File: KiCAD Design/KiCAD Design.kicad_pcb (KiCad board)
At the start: 2 copper layers, 51 x 60.5 mm, 60 parts, among them J1 USB_B_Micro, J2 Conn_01x04_Pin, J5 Micro_SD_Card, SW1 SW_SPDT, U1 STM32F103C8Tx, U2 AMS1117-3.3, U3 BNO055, U4 L80-R, U5 nRF24L01P, Y1 16MHz, Y2 16MHz

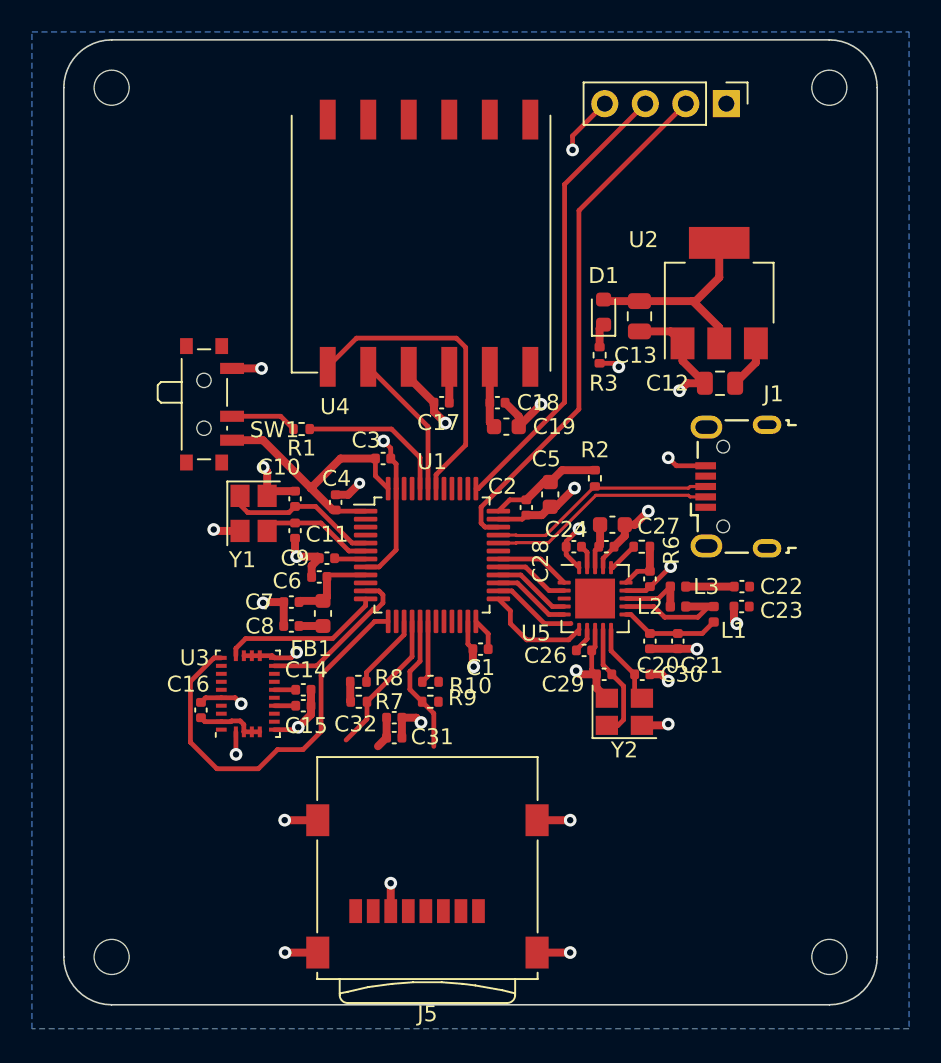
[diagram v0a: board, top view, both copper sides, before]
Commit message: All layout finished, ready to prep for order
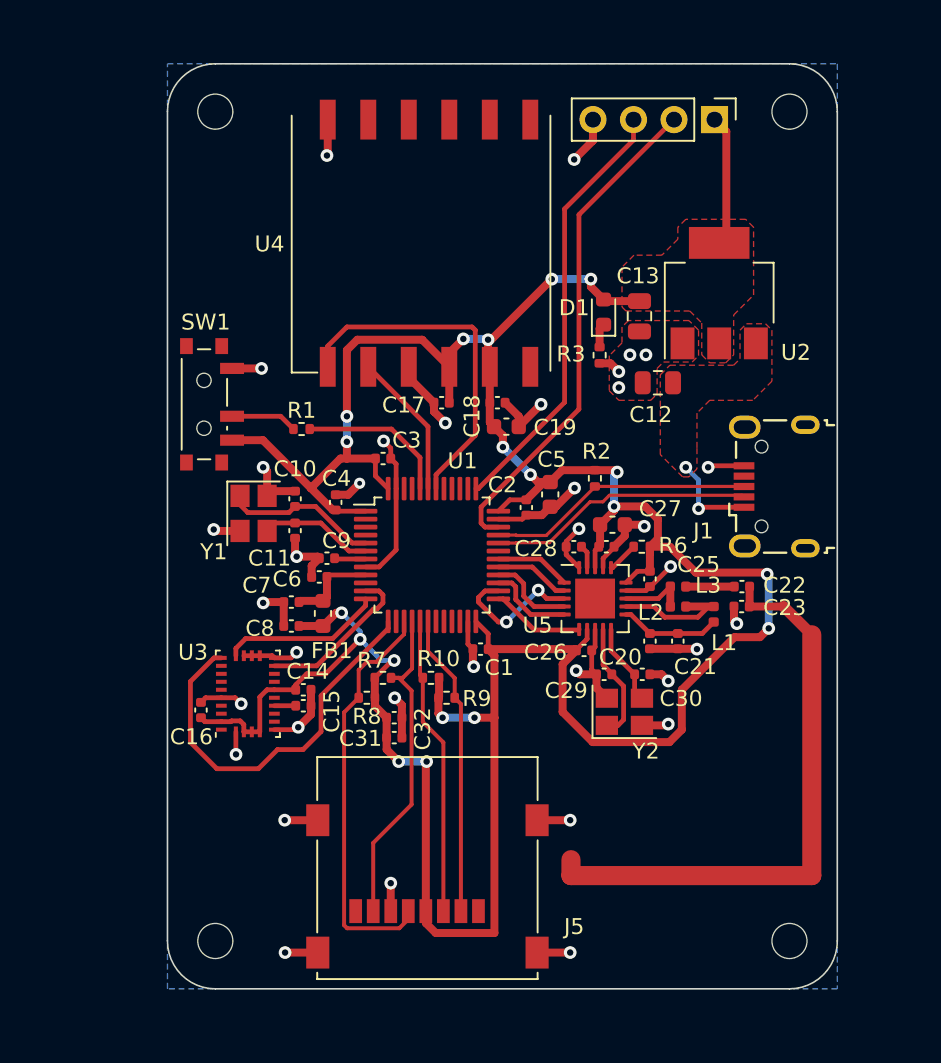
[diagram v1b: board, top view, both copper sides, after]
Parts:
- moved H1 6.67 mm to (146.2, 71.5)
- moved H3 6.58 mm to (146.2, 123.5)
- moved C12 3.90 mm to (174.0, 88.5)
- moved H2 2.92 mm to (182.2, 71.5)
- moved H4 2.69 mm to (182.2, 123.5)
- moved J1 2.41 mm to (181.3, 95.0)
- moved R7 2.13 mm to (156.8, 107.0)
- moved R9 1.50 mm to (159.8, 107.0)
- moved R10 1.42 mm to (160.8, 108.2), turned to 0 degrees
- moved J2 1.24 mm to (177.6, 72.0)
- moved R8 1.13 mm to (155.8, 108.2), turned to 180 degrees
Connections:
- J1 pad 6: unconnected-(J1-Shield-Pad6) -> (no net)
- U5 pad 21: GND -> (no net)
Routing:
- net +3.3V: track 64.2 -> 205.3 mm, vias 0 -> 19
- net Antenna: track 0.00 -> 37.1 mm
- net SPI1_SCK: track 4.76 -> 25.8 mm
- net SD_CD: track 3.94 -> 19.0 mm
- net SPI1_MISO: track 9.15 -> 20.9 mm
- net SPI1_MOSI: track 8.72 -> 18.8 mm
- net GND: track 107.6 -> 100.6 mm, vias 33 -> 36
- net SPI2_SCK: track 5.47 -> 8.65 mm, vias 0 -> 2
- net UART3_TX: track 19.3 -> 22.1 mm
- net VBUS: track 3.04 -> 5.82 mm, vias 0 -> 2
- net /USB_D+: track 14.3 -> 16.7 mm
- net /USB_D-: track 14.3 -> 16.7 mm
- net /SWDIO: track 32.8 -> 31.5 mm
- net /SWCLK: track 28.6 -> 27.3 mm
- net SPI2_IRQ: track 6.87 -> 5.88 mm
- added copper zone on F.Cu, net +3.3V
- added copper zone on F.Cu, net GND
- added copper zone on F.Cu, net VBUS
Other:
- board size 51 x 60.5 mm -> 42 x 58 mm
